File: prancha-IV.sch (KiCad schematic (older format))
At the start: 12 parts

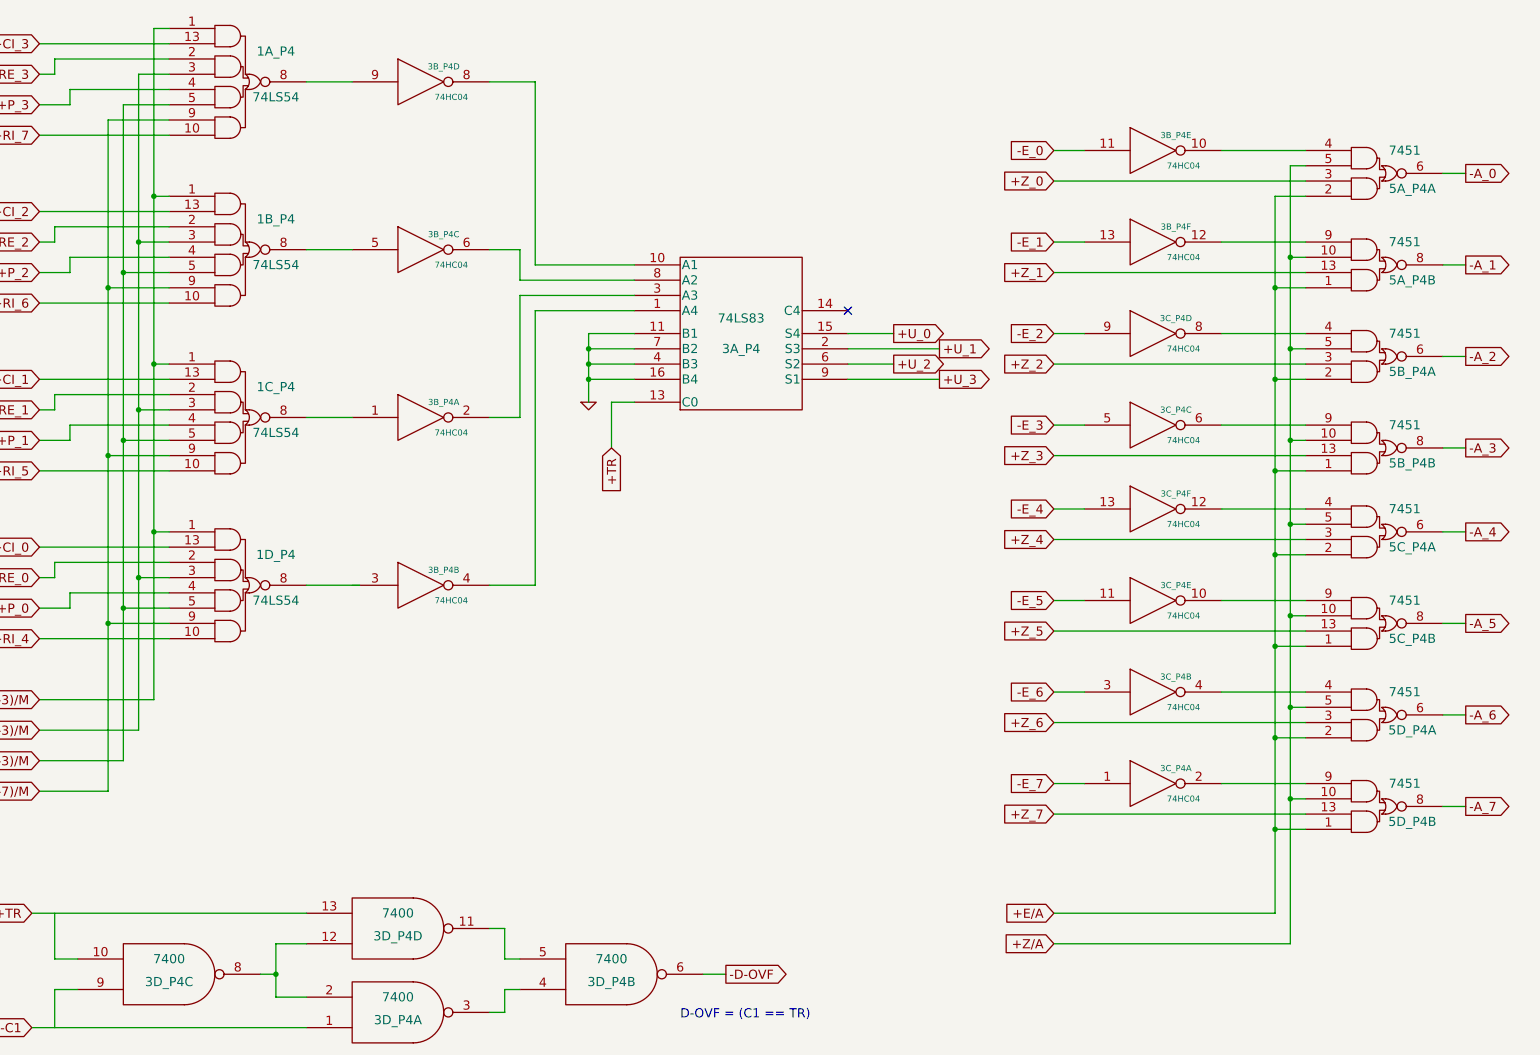
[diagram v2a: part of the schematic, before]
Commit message: wip
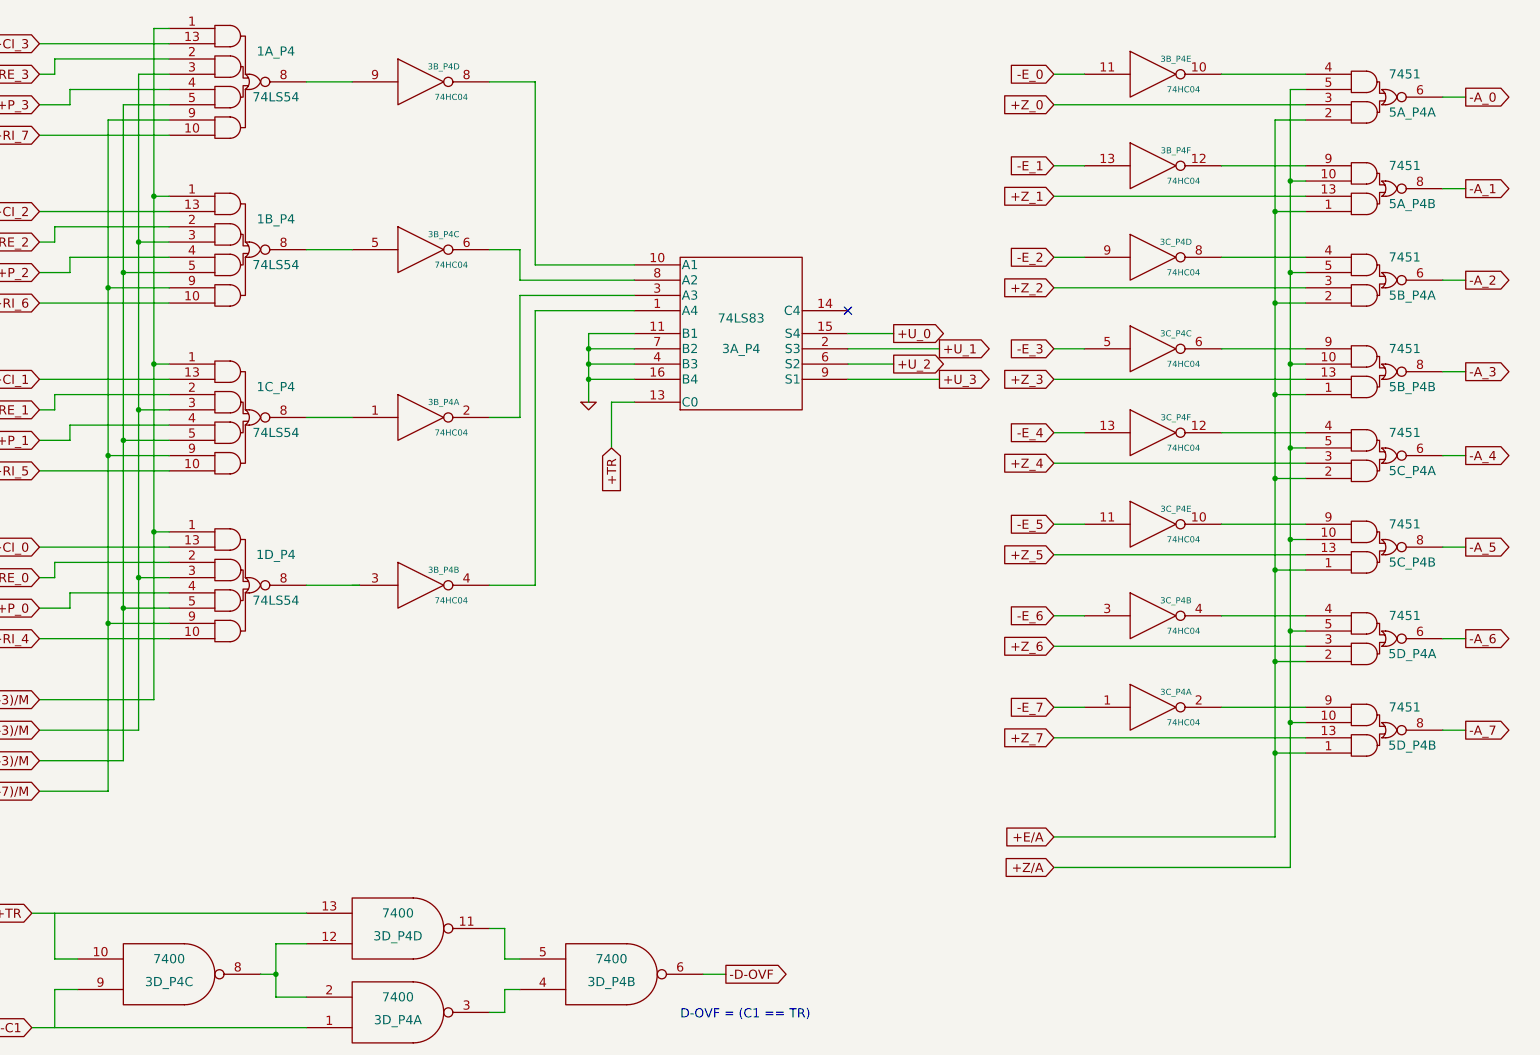
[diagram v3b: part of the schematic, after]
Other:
- moved on the sheet: 3B_P4E, 3B_P4F, 3C_P4A, 3C_P4B, 3C_P4C, 3C_P4D, 3C_P4E, 3C_P4F, 5A_P4A, 5A_P4B, 5B_P4A, 5B_P4B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

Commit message: redimensionando todas pranchas para tamanho A2
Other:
- moved on the sheet: 1A_P4, 1B_P4, 1C_P4, 1D_P4, 3A_P4, 3B_P4A, 3B_P4B, 3B_P4C, 3B_P4D, 3B_P4E, 3B_P4F, 3C_P4A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

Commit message: conector de 70 pinos para a interconexão das placas e término do desenho da prancha 5.
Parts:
- added P?: CONN_35X2, symbol CONN_35X2
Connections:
- new net ?: P?.1 (P1), P?.10 (P10), P?.11 (P11), P?.12 (P12), P?.13 (P13), P?.14 (P14), P?.15 (P15), P?.16 (P16), P?.17 (P17), P?.18 (P18), P?.19 (P19), P?.2 (P2), P?.20 (P20), P?.21 (P21), P?.22 (P22), P?.23 (P23), P?.24 (P24), P?.25, P?.26 (P26), P?.27 (P27), P?.28 (P28), P?.29 (P29), P?.3 (P3), P?.30 (P30), P?.31 (P31), P?.32 (P32), P?.33 (P33), P?.34 (P34), P?.35 (P35), P?.36 (P36), P?.37 (P37), P?.38 (P38), P?.39 (P39), P?.4 (P4), P?.40 (P40), P?.41 (P41), P?.42 (P42), P?.43 (P43), P?.44 (P44), P?.45 (P45), P?.46 (P46), P?.47 (P47), P?.48 (P48), P?.49 (P49), P?.5 (P5), P?.50 (P50), P?.51 (P51), P?.52 (P52), P?.53 (P53), P?.54 (P54), P?.55 (P55), P?.56 (P56), P?.57 (P57), P?.58 (P58), P?.59 (P59), P?.6 (P6), P?.60 (P60), P?.61 (P61), P?.62 (P62), P?.63 (P63), P?.64 (P64), P?.65 (P65), P?.66 (P66), P?.67 (P67), P?.68 (P68), P?.69 (P69), P?.7 (P7), P?.70 (P70), P?.8 (P8), P?.9 (P9)
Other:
- moved on the sheet: 1A_P4, 1B_P4, 1C_P4, 1D_P4, 3A_P4, 3B_P4A, 3B_P4B, 3B_P4C, 3B_P4D
